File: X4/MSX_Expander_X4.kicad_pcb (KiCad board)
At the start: 2 copper layers, 82.8 x 74.4 mm, 14 parts, among them J1 Conn_02x25_Odd_Even, J2 Conn_02x25_Odd_Even, J3 Conn_02x25_Odd_Even, U1 74LS21

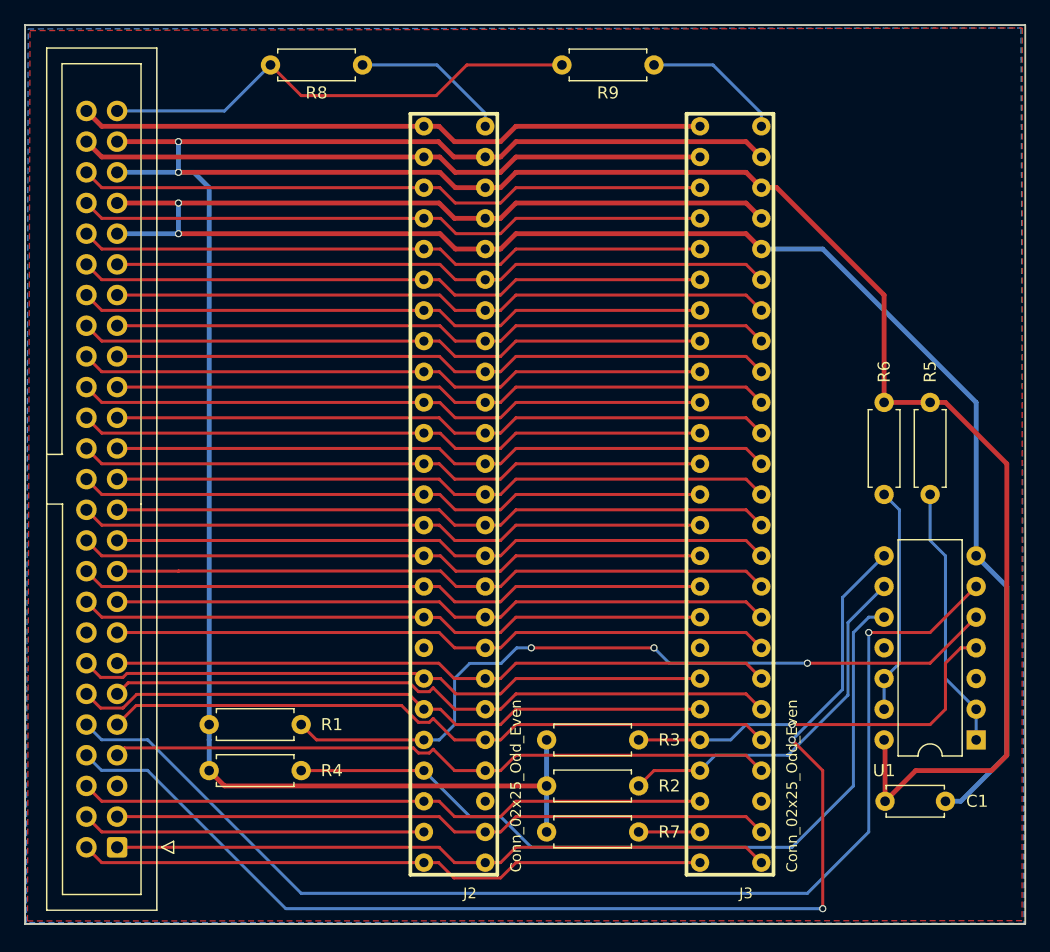
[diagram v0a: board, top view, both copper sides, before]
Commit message: routing pcb
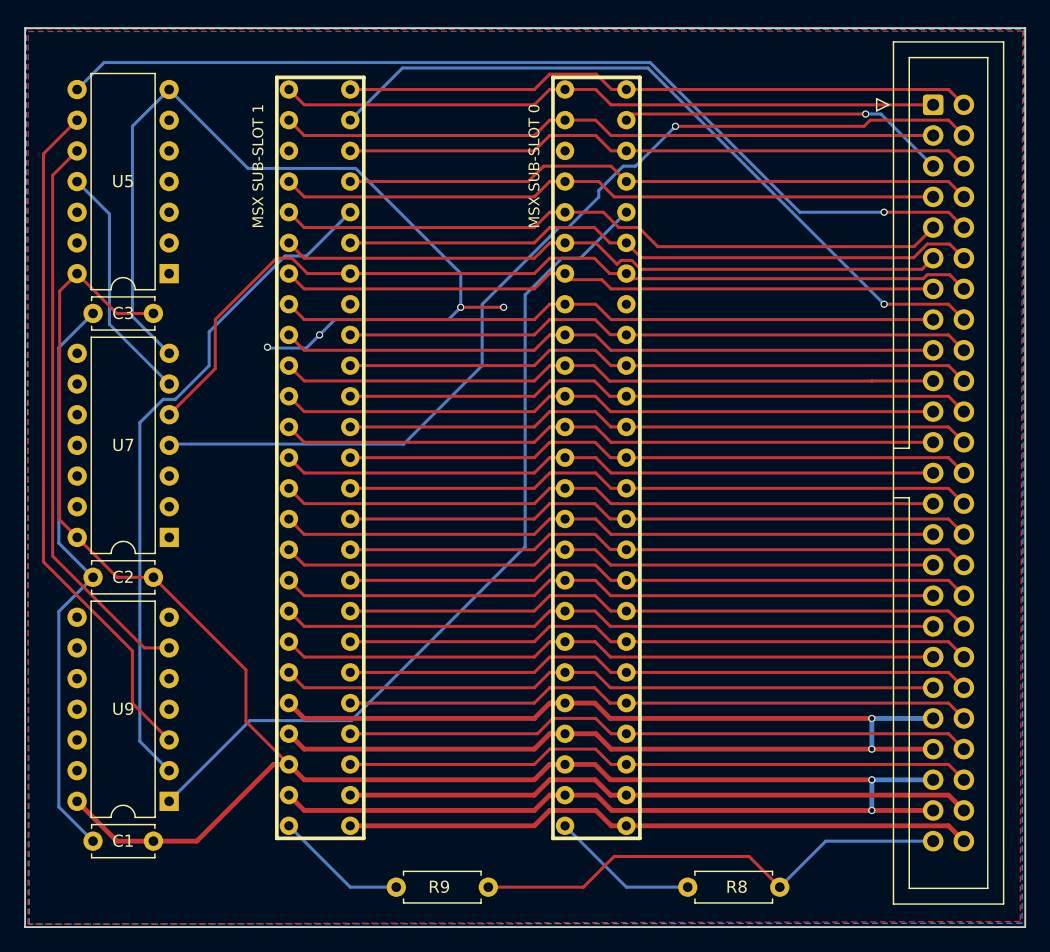
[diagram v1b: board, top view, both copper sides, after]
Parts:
- removed R1, R2, R3, R4, R5, R6, R7: 10K, Resistors_THT:R_Axial_DIN0207_L6.3mm_D2.5mm_P7.62mm_Horizontal
- removed U1: 74LS21, Housings_DIP:DIP-14_W7.62mm
- added C2: 0.1, Capacitor_THT:C_Disc_D5.0mm_W2.5mm_P5.00mm, F.Cu at (91.9, 119.9)
- added C3: 0.1, Capacitor_THT:C_Disc_D5.0mm_W2.5mm_P5.00mm, F.Cu at (91.9, 98.0)
- added U5: 74LS11, Package_DIP:DIP-14_W7.62mm, F.Cu at (93.2, 94.7)
- added U7: 74LS32, Package_DIP:DIP-14_W7.62mm, F.Cu at (93.2, 116.6)
- added U9: 74LS08, Package_DIP:DIP-14_W7.62mm, F.Cu at (93.2, 138.4)
- C1: footprint Capacitors_THT:C_Disc_D4.7mm_W2.5mm_P5.00mm -> Capacitor_THT:C_Disc_D5.0mm_W2.5mm_P5.00mm
- J1: value Conn_02x25_Odd_Even -> IDC50P - MSX BUS; footprint Roni Footprints:IDC-Header_2x25_P2.54mm_Vertical -> Connector_IDC:IDC-Header_2x25_P2.54mm_Vertical
- J2: value Conn_02x25_Odd_Even -> MSX SUB-SLOT 0
- J3: value Conn_02x25_Odd_Even -> MSX SUB-SLOT 1
- moved J1 91.3 mm to (156.5, 80.8), turned to 0 degrees
- moved J3 75.0 mm to (103.1, 79.5), turned to -90 degrees
- moved R8 73.2 mm to (136.1, 145.5), turned to 0 degrees
- moved R9 71.3 mm to (112.0, 145.5), turned to 0 degrees
- moved J2 64.3 mm to (126.0, 79.5), turned to -90 degrees
- moved C1 60.7 mm to (91.9, 141.7), turned to 180 degrees
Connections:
- net SOUND_A renamed SOUND0
- net SOUND_B renamed SOUND1
- J1 pad 16: unconnected-(J1-Pad16) -> EXP_SLTSL1
- J1 pad 5: unconnected-(J1-Pad5) -> EXP_SLTSL0
- J2 pad 10: /BUSDIR_A -> /BUSDIR0
- J2 pad 4: /SLTSL -> EXP_SLTSL0
- J2 pad 8: /INT_A -> /INT
- J3 pad 10: /BUSDIR_B -> /BUSDIR1
- J3 pad 4: Net-(J3-Pad4) -> EXP_SLTSL1
- J3 pad 8: /INT_B -> /INT
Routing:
- net +5V: track 275.7 -> 192.5 mm
- net /BUSDIR0: track 0.00 -> 70.3 mm
- net GND: track 172.3 -> 239.4 mm, vias 2 -> 6
- net /INT_A: track 66.2 -> 0.00 mm
- net /BUSDIR_A: track 63.9 -> 0.00 mm, vias 3 -> 0
- net EXP_SLTSL1: track 0.00 -> 61.2 mm, vias 0 -> 1
- net Net-(U5-Pad9): track 0.00 -> 56.8 mm
- net /BUSDIR1: track 0.00 -> 56.1 mm
- net /SLTSL: track 28.5 -> 80.8 mm, vias 0 -> 1
- net /INT: track 99.6 -> 52.4 mm, vias 2 -> 0
- net Net-(U5-Pad10): track 0.00 -> 47.2 mm
- net /BUSDIR_B: track 33.3 -> 0.00 mm, vias 1 -> 0
- net /INT_B: track 30.7 -> 0.00 mm
- net EXP_SLTSL0: track 0.00 -> 27.4 mm, vias 0 -> 1
- net /RD: track 52.7 -> 75.9 mm
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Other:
- outline, holes or cut-outs redrawn
